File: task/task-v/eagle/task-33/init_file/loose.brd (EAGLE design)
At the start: 54.3 x 38.1 mm, 12 parts, among them IC1 16F84, U1 78L05

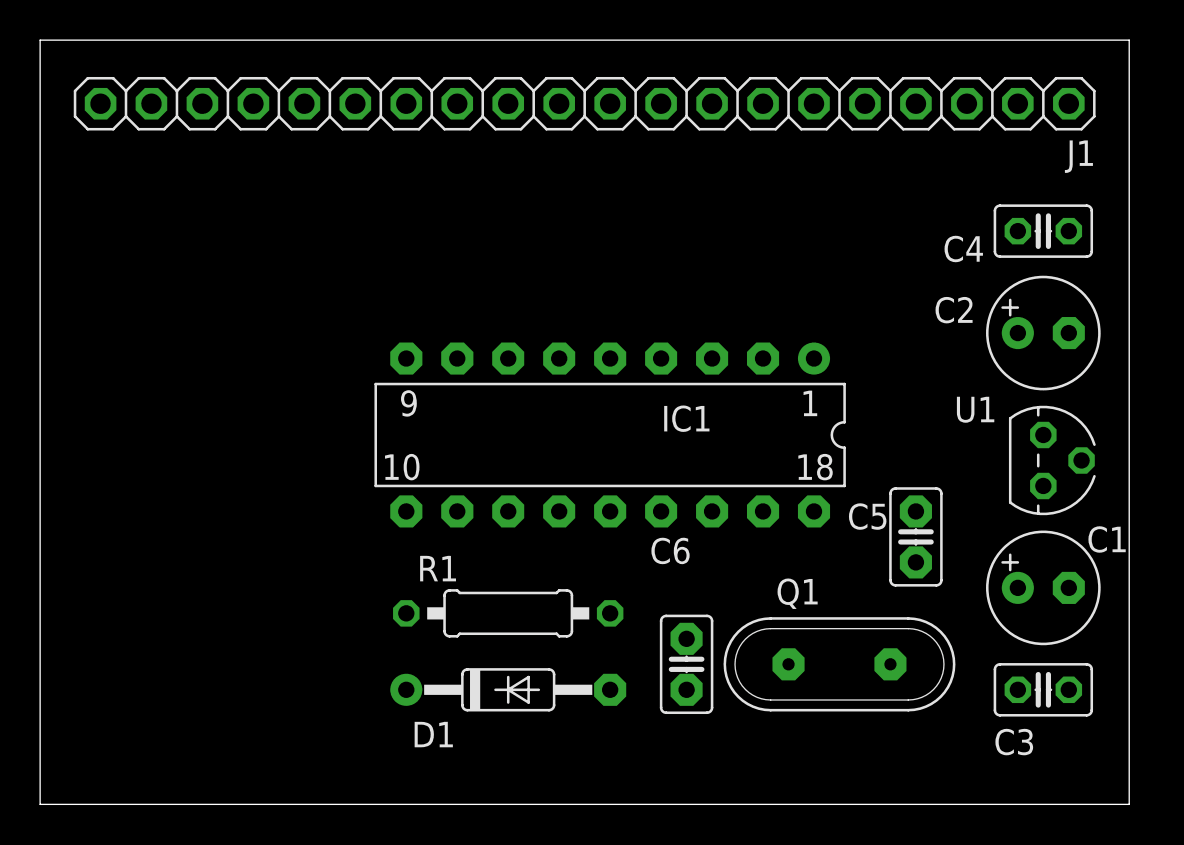
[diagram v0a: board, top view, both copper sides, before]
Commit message: Refine engineering task metadata and instructions
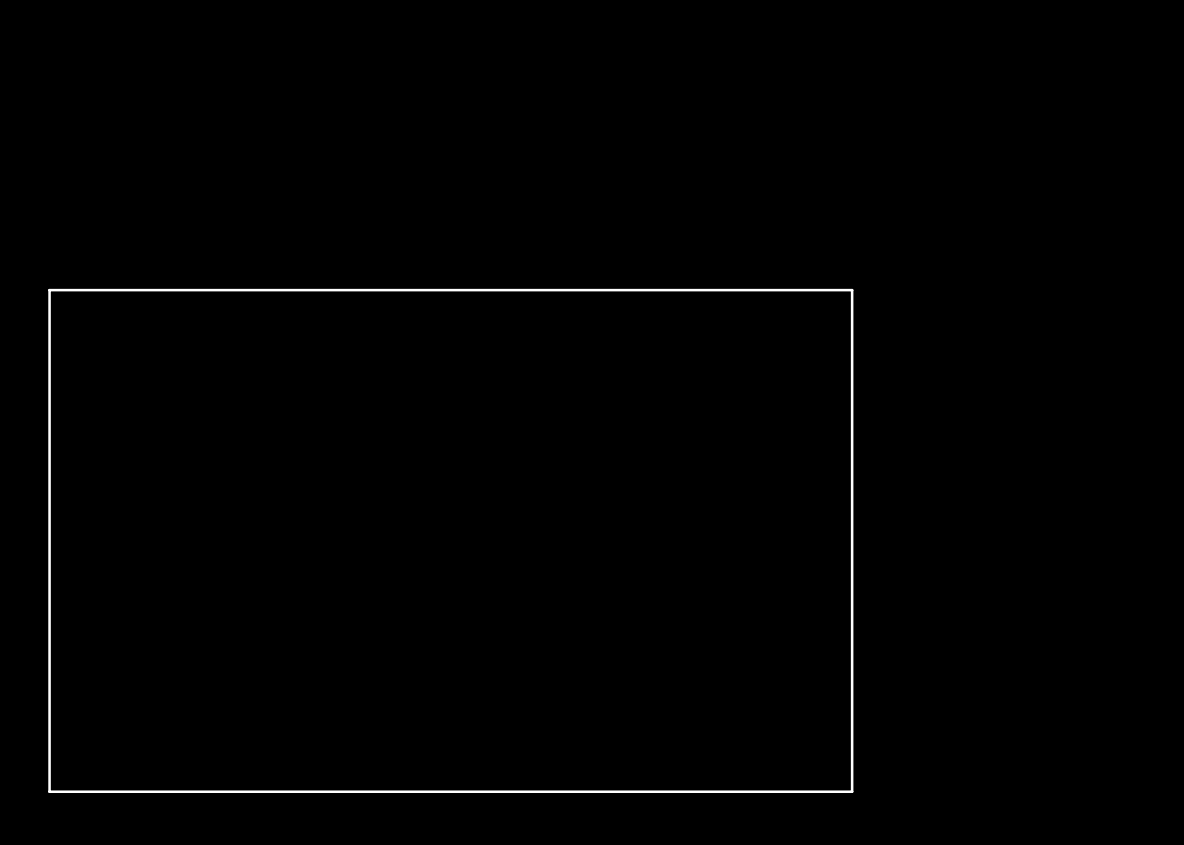
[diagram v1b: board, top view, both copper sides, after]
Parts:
- removed C1, C2: 10u, polcap:E2,5-6
- removed C3, C4: 10n, rcl:C025-025X050
- removed C5, C6: 27p, capacitor-wima:C2,5-2
- removed D1: 1N4148, diode:DO35-10
- removed IC1: 16F84, microchip:DIL18
- removed J1: (no value), PINHEAD:1X20
- removed Q1: (no value), special:QS
- removed R1: 2.2k, rcl:0207/10
- removed U1: 78L05, linear:TO92
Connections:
- removed net +12V: C1.+, C3.2, J1.2, U1.3
- removed net A0: IC1.17, J1.4
- removed net A1: IC1.18, J1.5
- removed net A2: IC1.1, J1.6
- removed net A3: IC1.2, J1.7
- removed net A4: IC1.3, J1.8
- removed net B0: IC1.6, J1.9
- removed net B1: IC1.7, J1.10
- removed net B2: IC1.8, J1.11
- removed net B3: IC1.9, J1.12
- removed net B4: IC1.10, J1.13
- removed net B5: IC1.11, J1.14
- removed net B6: IC1.12, J1.15, J1.18
- removed net B7: IC1.13, J1.16, J1.17
- removed net GND: C1.-, C2.-, C3.1, C4.1, C5.1, C6.1, IC1.5, J1.1, J1.20, U1.2
- removed net N$1: D1.K, IC1.4, J1.19
- removed net N$2: D1.A, R1.1
- removed net N$3: C5.2, IC1.16, Q1.2
- removed net N$4: C6.2, IC1.15, Q1.1
- removed net VCC: C2.+, C4.2, IC1.14, J1.3, R1.2, U1.1
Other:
- board size 54.3 x 38.1 mm -> 40 x 25 mm
